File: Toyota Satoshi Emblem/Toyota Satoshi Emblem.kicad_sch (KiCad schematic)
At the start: 293 parts

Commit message: v1.1
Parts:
- removed D? (x58): W_LED, symbol Device:LED
- removed J?: Conn_01x20_Male, symbol Connector:Conn_01x20_Male
- removed Q? (x6): BC337, Package_TO_SOT_THT:TO-92_Inline, symbol Transistor_BJT:BC337
- removed Q? (x12): BC327, Package_TO_SOT_THT:TO-92_Inline, symbol Transistor_BJT:BC327
- removed R? (x29): 10Ω, symbol Device:R
- removed R? (x12): 10KΩ, symbol Device:R
- removed R? (x12): 200Ω, symbol Device:R
- added D? (x86): A_LED, symbol Device:LED
- added Q? (x6): BC327, Package_TO_SOT_THT:TO-92_Inline, symbol Transistor_BJT:BC327
- added Q? (x12): S8550, Package_TO_SOT_THT:TO-92_Inline, symbol Transistor_BJT:S8550
- added R? (x86): 9Ω, symbol Device:R
- added R? (x12): 200Ω, symbol Device:R
- added R? (x12): 10KΩ, symbol Device:R
- added U? (x7): 74HC04, symbol 74xx:74HC04
- R?: value 200Ω -> 7.5k
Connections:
- net +5V: now also R?.2, R?.2, R?.2, R?.2, R?.2, R?.2, R?.2, R?.2, R?.2, R?.2, R?.2, R?.2
- net BUCK_A: now also Q?.3 (E), Q?.3 (E), Q?.3 (E)
- net BUCK_B: now also Q?.3 (E), Q?.3 (E), Q?.3 (E)
- net GND: now also D?.1 (K), D?.1 (K), D?.1 (K), D?.1 (K), D?.1 (K), D?.1 (K), D?.1 (K), D?.1 (K), D?.1 (K), D?.1 (K), D?.1 (K), D?.1 (K), D?.1 (K), D?.1 (K), D?.1 (K), D?.1 (K), D?.1 (K), D?.1 (K), D?.1 (K), D?.1 (K), D?.1 (K), D?.1 (K), D?.1 (K), D?.1 (K), D?.1 (K), D?.1 (K), D?.1 (K), D?.1 (K), D?.1 (K), D?.1 (K), D?.1 (K), D?.1 (K), D?.1 (K), D?.1 (K), D?.1 (K), D?.1 (K), D?.1 (K), D?.1 (K), D?.1 (K), D?.1 (K), D?.1 (K), D?.1 (K), D?.1 (K), D?.1 (K), D?.1 (K), D?.1 (K), D?.1 (K), D?.1 (K), D?.1 (K), D?.1 (K), D?.1 (K), D?.1 (K), D?.1 (K), D?.1 (K), D?.1 (K), D?.1 (K), D?.1 (K), D?.1 (K), D?.1 (K), D?.1 (K), D?.1 (K), D?.1 (K), D?.1 (K), D?.1 (K), D?.1 (K), D?.1 (K), D?.1 (K), D?.1 (K), D?.1 (K), D?.1 (K), D?.1 (K), D?.1 (K), R?.1, R?.1, R?.1, R?.1, R?.1, R?.1; no longer R?.2, R?.2, R?.2, R?.2, R?.2, R?.2
- net at R?.1, R?.1, R?.1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: now also Q?.3 (C)
- net at R?.2: now also U?.4
- net at R?.1, R?.1, R?.1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: now also Q?.3 (C) (x2)
- net at R?.1, R?.1: now also Q?.2 (B) (x6)
- net at R?.1, R?.1, R?.1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: now also Q?.3 (C), R?.1
- net at R?.1, R?.1, R?.1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: now also Q?.3 (C), R?.1, R?.1 (x2)
- net at R?.2: now also U?.6
- net at R?.2: now also U?.8
- net at R?.2: now also U?.2
- net at R?.2: now also U?.12
- net at R?.2: now also U?.10
- new net: D?.1 (K), D?.2 (A) (x43)
- new net: D?.2 (A), R?.2 (x43)
- new net: R?.2, U?.3
- new net: R?.1, R?.2 (x43)
- new net: Q?.2 (B), R?.2, R?.2 (x6)
- new net: Q?.1 (E), Q?.1 (E) (x6)
- new net: Q?.2 (B), R?.1, R?.1 (x6)
- new net: Q?.3 (C), R?.1, R?.1, R?.1, R?.1, R?.1, R?.1 (x5)
- new net: R?.2, U?.9
- new net: R?.2, U?.1
- new net: R?.2, U?.11
- new net: R?.2, U?.5
- new net: Q?.3 (C), R?.1, R?.1, R?.1, R?.1
- new net: R?.2, U?.13
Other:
- note removed: "WHITE"
- note removed: "WHITE TOGGLE"
- moved on the sheet: D?, R?

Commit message: v1.2
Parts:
- removed Q? (x6): BC327, Package_TO_SOT_THT:TO-92_Inline, symbol Transistor_BJT:BC327
- removed Q? (x12): S8550, Package_TO_SOT_THT:TO-92_Inline, symbol Transistor_BJT:S8550
- removed R? (x17): 200Ω, symbol Device:R
- removed R? (x36): 9Ω, symbol Device:R
- removed R? (x18): 10KΩ, symbol Device:R
- removed R?: 7.5k, symbol Device:R
- removed U? (x7): 74HC04, symbol 74xx:74HC04
- added Q? (x6): 2N3904, Package_TO_SOT_THT:TO-92_Inline, symbol Transistor_BJT:2N3904
- added Q? (x18): IRLZ44N, Package_TO_SOT_THT:TO-220-3_Vertical, symbol Transistor_FET:IRLZ44N
- added R? (x12): 10K, symbol Device:R
- added R? (x6): 200, symbol Device:R
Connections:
- net at R?.1, R?.1, R?.1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: now also R?.1, R?.1, Q?.2 (D) (x2)
- net at R?.2: now also D?.2 (A) (x26)
- net at D?.2 (A): now also R?.2 (x10)
- net at R?.1, R?.1, R?.1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: now also Q?.2 (D) (x10)
- new net: Q?.1 (G), Q?.3 (C), R?.1 (x6)
- new net: R?.2, R?.2 (x3)
- new net: Q?.1 (E), Q?.3 (S), R?.2 (x6)
- new net: Q?.2 (B), R?.1 (x6)
- new net: Q?.2 (D), Q?.3 (S), Q?.3 (S) (x6)
- new net: Q?.1 (G), R?.1, R?.2 (x6)
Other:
- note removed: "AMBER TOGGLE"
- note removed: "LETTER INTENSITY"
- moved on the sheet: D?, R?

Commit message: v1.3
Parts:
- removed D? (x120): A_LED, symbol Device:LED
- removed J?: Conn_01x20_Female, symbol Connector:Conn_01x20_Female
- removed R? (x90): 9Ω, symbol Device:R
- added C?: 200uF, symbol Device:C_Polarized
- added C?: 100uF, symbol Device:C_Polarized
- added D? (x120): A_LED, symbol Device:LED
- added D?: 1N5822, Diode_THT:D_DO-201AD_P15.24mm_Horizontal, symbol Diode:1N5822
- added J? (x6): Conn_01x03_Male, symbol Connector:Conn_01x03_Male
- added J? (x6): Letter Terminal, symbol Connector:Conn_01x03_Female
- added L?: 68uH, symbol Device:L
- added R? (x2): R, symbol Device:R
- added R? (x90): 9Ω, symbol Device:R
- added U?: LM2596S-ADJ, Package_TO_SOT_SMD:TO-263-5_TabPin3, symbol Regulator_Switching:LM2596S-ADJ
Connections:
- net BUCK_A: now also R?.2, R?.2, J?.2 (Pin_2), J?.2 (Pin_2)
- net BUCK_B: now also R?.2, R?.2, J?.2 (Pin_2), J?.2 (Pin_2)
- net GND: now also Q?.1 (E), Q?.1 (E), Q?.1 (E), Q?.1 (E), Q?.1 (E), Q?.1 (E), Q?.3 (S), Q?.3 (S), Q?.3 (S), Q?.3 (S), Q?.3 (S), Q?.3 (S), R?.2, R?.2, R?.2, R?.2, R?.2, R?.2, C?.2, C?.2, D?.2 (A), R?.1, U?.3 (GND); no longer A?.4 (GND), D?.1 (K), D?.1 (K), D?.1 (K), D?.1 (K), D?.1 (K), D?.1 (K), D?.1 (K), D?.1 (K), D?.1 (K), D?.1 (K), D?.1 (K), D?.1 (K)
- net VDD: now also C?.1, U?.1 (VIN)
- net at Q?.2 (D): now also J?.1 (Pin_1) (x5)
- net BUCK_C: now reaches R?.2, R?.2
- net BUCK_C: now also C?.1, J?.2 (Pin_2), J?.2 (Pin_2), L?.2, R?.1
- net at Q?.1 (G): now also A?.13 (D10)
- net at Q?.1 (G), R?.1, R?.2: now also A?.11 (D8)
- net at R?.1, R?.1, R?.1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: now also R?.1, R?.1, R?.1, R?.1, R?.1, R?.1, J?.2 (Pin_2); no longer Q?.2 (D)
- net at Q?.1 (G), R?.1, R?.2: now also A?.5 (D2)
- net at Q?.2 (D): now also J?.3 (Pin_3) (x5)
- net at Q?.1 (G): now also A?.6 (D3)
- net at A?.15 (D12): now also Q?.1 (G), R?.1, R?.2
- net at A?.16 (D13): now also Q?.1 (G), R?.1, R?.2
- net at A?.8 (D5): now also Q?.1 (G)
- net at A?.9 (D6): now also Q?.1 (G)
- net at A?.12 (D9): now also Q?.1 (G)
- net at A?.14 (D11): now also Q?.1 (G)
- net at A?.7 (D4): now also Q?.1 (G), R?.1, R?.2
- net at A?.10 (D7): now also Q?.1 (G), R?.1, R?.2
- new net: D?.1 (K), D?.2 (A) (x60)
- new net: D?.2 (A), R?.2 (x60)
- new net: D?.1 (K), D?.1 (K), D?.1 (K), D?.1 (K), D?.1 (K), D?.1 (K), J?.1 (Pin_1) (x6)
- new net: J?.2 (Pin_2), R?.1, R?.1, R?.1, R?.1, R?.1, R?.1, R?.1, R?.1, R?.1, R?.1, R?.1, R?.1 (x5)
- new net: D?.1 (K), D?.1 (K), D?.1 (K), D?.1 (K), D?.1 (K), D?.1 (K), J?.3 (Pin_3) (x6)
- new net: R?.2, R?.2, U?.4 (FB)
- new net: R?.1, R?.2 (x30)
- new net: J?.1 (Pin_1), Q?.2 (D)
- new net: J?.3 (Pin_3), Q?.2 (D)
- new net: D?.1 (K), L?.1, U?.2 (OUT)
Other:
- note removed: "AMBER"
- moved on the sheet: 5A, 6A10, A?, C?, D?, L?, Q?, R?, U?

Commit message: v1.4
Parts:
- removed Q?: BC327, Package_TO_SOT_THT:TO-92_Inline, symbol Transistor_BJT:BC327
- removed R? (x60): 9Ω, symbol Device:R
- added C?: 0.22u, symbol Device:C
- added D? (x4): 1N47xxA, Diode_THT:D_DO-41_SOD81_P10.16mm_Horizontal, symbol Diode:1N47xxA
- added J?: Power Port Terminal, symbol Connector_Generic:Conn_02x04_Counter_Clockwise
- added J? (x2): Serial Terminal, symbol Connector:Conn_01x02_Male
- added J?: Ambient Harness, symbol Connector:Conn_01x02_Female
- added K?: FINDER-40.51, Relay_THT:Relay_SPDT_Finder_40.51, symbol Relay:FINDER-40.51
- added Q?: BC337, Package_TO_SOT_THT:TO-92_Inline, symbol Transistor_BJT:BC337
- added R? (x60): 8.2, symbol Device:R
- added R? (x7): 10K, symbol Device:R
- added R?: R_Photo, symbol Device:R_Photo
- added R? (x4): 1K, symbol Device:R
- C?: value C_Polarized -> 10u
- C?: value C_Polarized -> 4.7u
- C?: value C -> 0.1u
- D?: value 5KPxxA -> 5KP16A
- F?: renamed from 5A; value Fuse -> 7.5A
- L? (x3): value 68uH -> 47uH
- R? (x12): value 9Ω -> 8.2
- R? (x36): value 9Ω -> 3.3
- R?: value R -> 1K
- R? (x6): value 200 -> 1K
- R? (x2): value R -> 3.3K
- R?: value R -> 4.7K
- R? (x2): value R -> 1.5K
- R?: value R -> 10K
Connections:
- net +5VD is gone; now on net +5V: C?.1, C?.1, U?.3 (OUT)
- net VDD is gone; now on net +12V: C?.1, C?.1, C?.1, U?.1 (VIN), U?.1 (VIN), U?.1 (VIN)
- net BUCK_A: now also J?.1 (Pin_1), R?.2, R?.2
- net BUCK_B: now also J?.2 (Pin_2), R?.2, R?.2
- net BUCK_C: now also J?.8 (Pin_8), R?.2, R?.2
- net GND: now also A?.29 (GND), C?.2, D?.2 (A), D?.2 (A), D?.2 (A), D?.2 (A), J?.1 (Pin_1), J?.4 (Pin_4), J?.5 (Pin_5), K?.A1
- net at D?.2 (A): now also R?.2 (x30)
- net at J?.2 (Pin_2), R?.1, R?.1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: now also R?.1, R?.1, R?.1, R?.1, R?.1, R?.1 (x5)
- net at A?.13 (D10), Q?.1 (G): now also R?.1
- net at 6A10.1 (K), C?.1, D?.1 (A1)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: now also C?.1, Q?.1 (C)
- net at A?.6 (D3), Q?.1 (G): now also R?.1
- net at F?.1: now also 6A10.2 (A)
- net at F?.2: now also K?.14; no longer 6A10.2 (A)
- net at A?.12 (D9), Q?.1 (G): now also R?.1
- net at R?.2: now also Q?.2 (B)
- net at D?.2 (A): now also Q?.3 (E)
- net at A?.9 (D6), Q?.1 (G): now also R?.1
- net at A?.1 (D1/TX): now also J?.2 (Pin_2)
- net at A?.14 (D11), Q?.1 (G): now also R?.1
- net at A?.2 (D0/RX): now also D?.1 (K), R?.1
- net at A?.23 (A4): now also D?.1 (K), R?.2
- net at A?.24 (A5): now also D?.1 (K), R?.2
- net at A?.25 (A6): now also D?.1 (K), R?.2
- net at A?.26 (A7): now also J?.2 (Pin_2), R?.2
- net +5V: now reaches A?.27 (+5V)
- net +5V: now also J?.7 (Pin_7), R?.1
- net at A?.8 (D5), Q?.1 (G): now also R?.1
- net VD renamed +12V
- net +12V: now also J?.3 (Pin_3), J?.6 (Pin_6)
- new net: R?.1, R?.2 (x30)
- new net: J?.1 (Pin_1), R?.1
- new net: J?.2 (Pin_2), R?.2
- new net: J?.1 (Pin_1), R?.2
- new net BAT +12V: K?.11
- new net HEAD RLY (R-B): K?.A2
- new net L Turn Sig: R?.1
- new net R Turn Sig: R?.1
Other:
- note added: "VEHICLE POWER ----->"
- moved on the sheet: 6A10, A?, C?, D?, F?, J?, L?, Q?, R?, U?

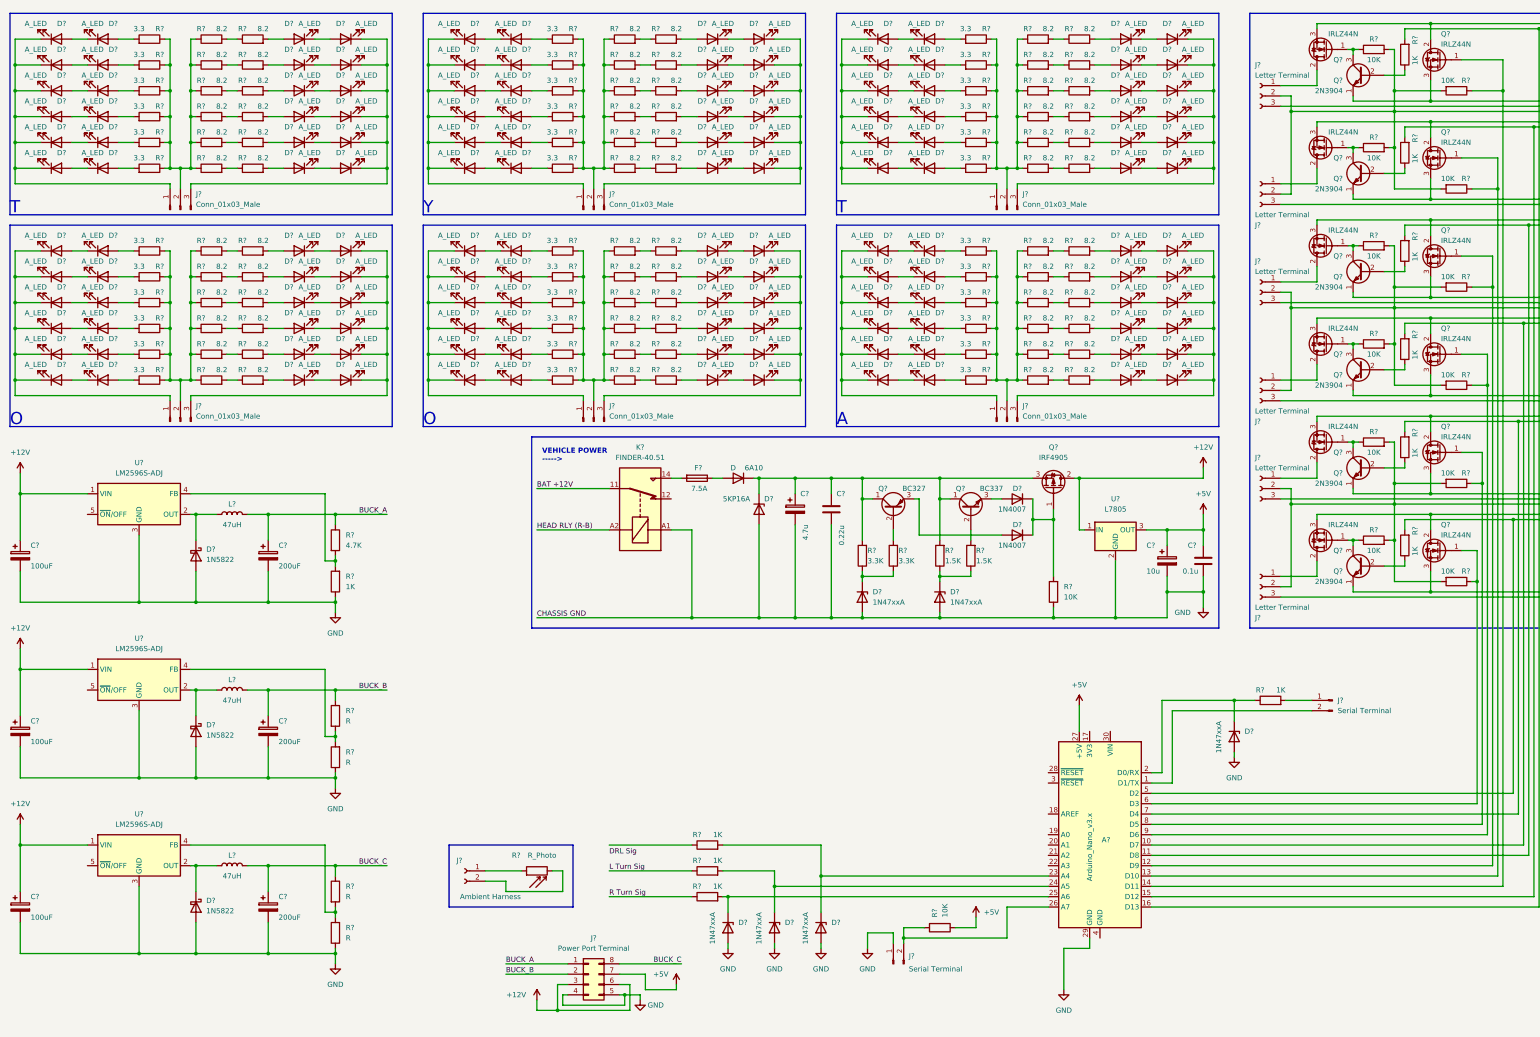
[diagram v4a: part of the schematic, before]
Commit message: v1.5
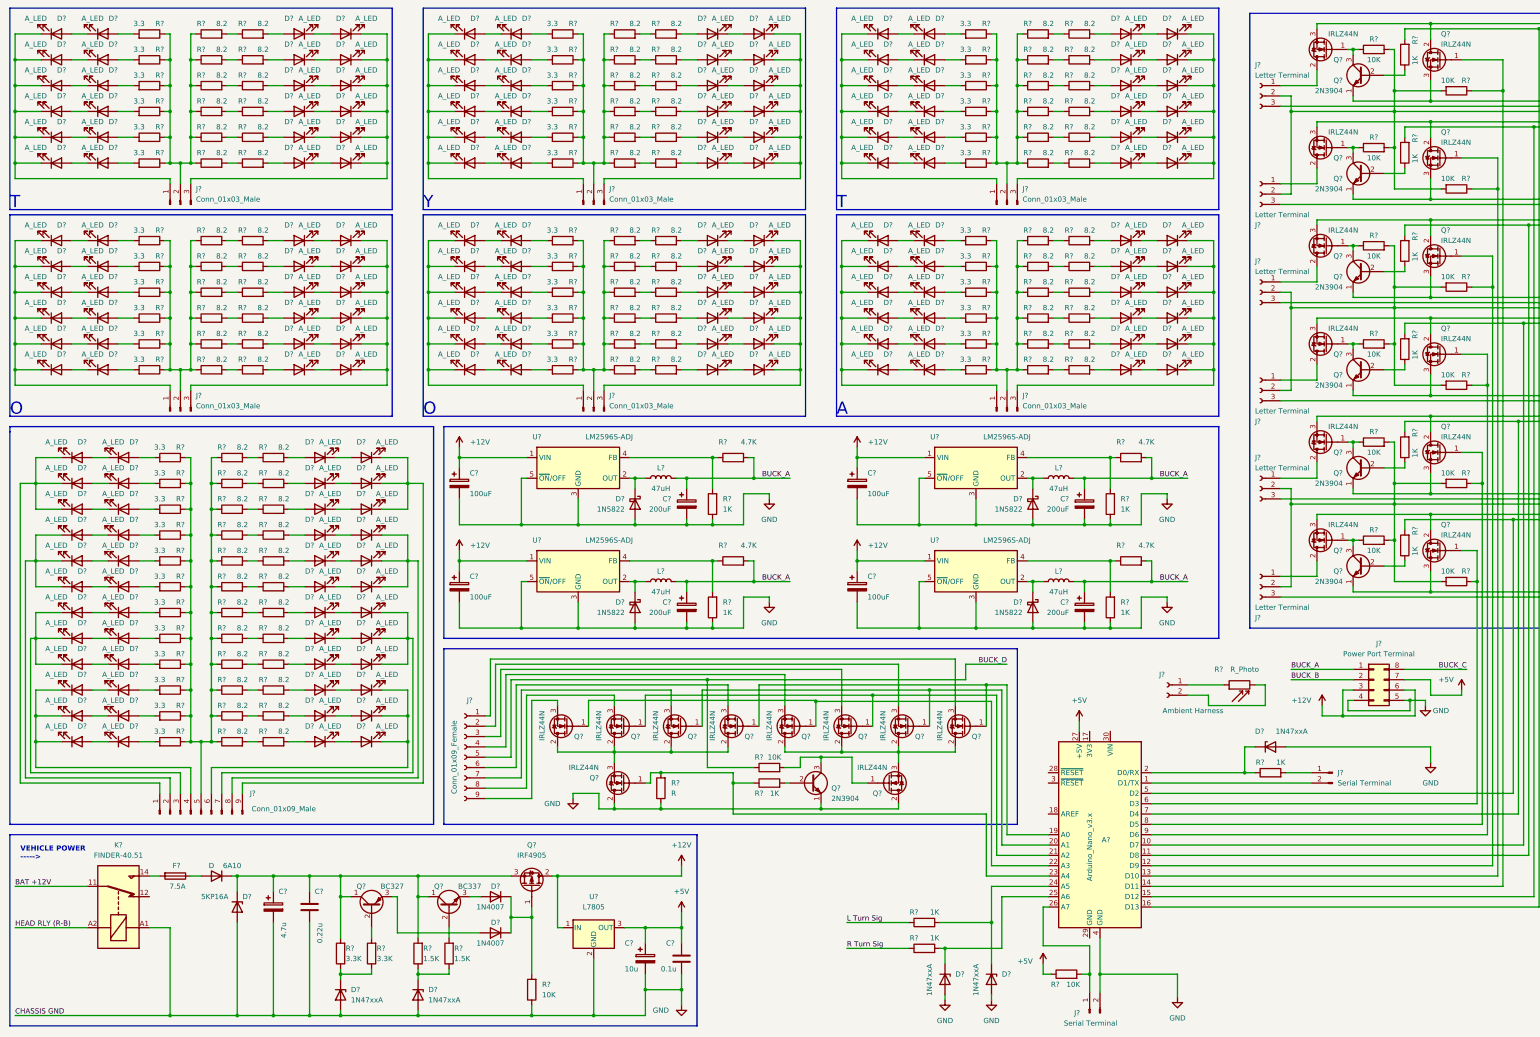
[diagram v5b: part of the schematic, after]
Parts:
- removed C? (x3): 200uF, symbol Device:C_Polarized
- removed C? (x3): 100uF, symbol Device:C_Polarized
- removed D?: 1N47xxA, Diode_THT:D_DO-41_SOD81_P10.16mm_Horizontal, symbol Diode:1N47xxA
- removed D? (x3): 1N5822, Diode_THT:D_DO-201AD_P15.24mm_Horizontal, symbol Diode:1N5822
- removed L? (x3): 47uH, symbol Device:L
- removed R? (x4): R, symbol Device:R
- removed R? (x2): 1K, symbol Device:R
- removed R?: 4.7K, symbol Device:R
- removed U? (x3): LM2596S-ADJ, Package_TO_SOT_SMD:TO-263-5_TabPin3, symbol Regulator_Switching:LM2596S-ADJ
- added C? (x4): 200uF, symbol Device:C_Polarized
- added C? (x4): 100uF, symbol Device:C_Polarized
- added D? (x48): A_LED, symbol Device:LED
- added D? (x4): 1N5822, Diode_THT:D_DO-201AD_P15.24mm_Horizontal, symbol Diode:1N5822
- added J?: Conn_01x09_Male, symbol Connector:Conn_01x09_Male
- added J?: Conn_01x09_Female, symbol Connector:Conn_01x09_Female
- added L? (x4): 47uH, symbol Device:L
- added Q?: 2N3904, Package_TO_SOT_THT:TO-92_Inline, symbol Transistor_BJT:2N3904
- added Q? (x10): IRLZ44N, Package_TO_SOT_THT:TO-220-3_Vertical, symbol Transistor_FET:IRLZ44N
- added R? (x24): 8.2, symbol Device:R
- added R? (x12): 3.3, symbol Device:R
- added R?: 10K, symbol Device:R
- added R? (x5): 1K, symbol Device:R
- added R?: R, symbol Device:R
- added R? (x4): 4.7K, symbol Device:R
- added U? (x4): LM2596S-ADJ, Package_TO_SOT_SMD:TO-263-5_TabPin3, symbol Regulator_Switching:LM2596S-ADJ
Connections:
- net +12V: now also C?.1, C?.1, C?.1, C?.1, U?.1 (VIN), U?.1 (VIN), U?.1 (VIN), U?.1 (VIN)
- net BUCK_A: now also C?.1, C?.1, C?.1, C?.1, L?.2, L?.2, L?.2, L?.2, R?.2, R?.2, R?.2, R?.2
- net GND: now also A?.4 (GND), J?.2 (Pin_2), C?.2, C?.2, C?.2, C?.2, C?.2, C?.2, C?.2, C?.2, D?.2 (A), D?.2 (A), D?.2 (A), D?.2 (A), Q?.1 (E), Q?.2 (D), Q?.2 (D), R?.1, R?.1, R?.1, R?.1, R?.1, U?.3 (GND), U?.3 (GND), U?.3 (GND), U?.3 (GND), U?.5 (~{ON}/OFF), U?.5 (~{ON}/OFF), U?.5 (~{ON}/OFF), U?.5 (~{ON}/OFF); no longer A?.29 (GND), J?.1 (Pin_1)
- net at A?.23 (A4): now also Q?.1 (G), R?.1, R?.2
- net at A?.26 (A7), R?.2: now also J?.1 (Pin_1); no longer J?.2 (Pin_2)
- net at A?.19 (A0): now also Q?.1 (G), Q?.1 (G)
- net at A?.20 (A1): now also Q?.1 (G), Q?.1 (G)
- net at A?.21 (A2): now also Q?.1 (G), Q?.1 (G)
- net at A?.22 (A3): now also Q?.1 (G), Q?.1 (G)
- new net: R?.1, R?.2 (x12)
- new net: D?.2 (A), R?.2 (x24)
- new net: D?.1 (K), L?.1, U?.2 (OUT) (x4)
- new net: R?.1, R?.2, U?.4 (FB) (x4)
- new net: D?.1 (K), D?.1 (K), D?.1 (K), J?.1 (Pin_1)
- new net: D?.1 (K), D?.2 (A) (x24)
- new net: J?.5 (Pin_5), R?.1, R?.1, R?.1, R?.1, R?.1, R?.1, R?.1, R?.1, R?.1, R?.1, R?.1, R?.1, R?.1, R?.1, R?.1, R?.1, R?.1, R?.1, R?.1, R?.1, R?.1, R?.1, R?.1, R?.1
- new net: D?.1 (K), D?.1 (K), D?.1 (K), J?.2 (Pin_2)
- new net: D?.1 (K), D?.1 (K), D?.1 (K), J?.3 (Pin_3)
- new net: D?.1 (K), D?.1 (K), D?.1 (K), J?.4 (Pin_4)
- new net: D?.1 (K), D?.1 (K), D?.1 (K), J?.6 (Pin_6)
- new net: D?.1 (K), D?.1 (K), D?.1 (K), J?.7 (Pin_7)
- new net: D?.1 (K), D?.1 (K), D?.1 (K), J?.8 (Pin_8)
- new net: D?.1 (K), D?.1 (K), D?.1 (K), J?.9 (Pin_9)
- new net: Q?.1 (G), Q?.3 (C), R?.2
- new net: Q?.2 (B), R?.2
- new net: Q?.2 (D), Q?.2 (D), Q?.2 (D), Q?.2 (D), Q?.3 (S) (x2)
- new net: J?.7 (Pin_7), Q?.3 (S)
- new net: J?.1 (Pin_1), Q?.3 (S)
- new net: J?.3 (Pin_3), Q?.3 (S)
- new net: J?.8 (Pin_8), Q?.3 (S)
- new net: J?.4 (Pin_4), Q?.3 (S)
- new net: J?.2 (Pin_2), Q?.3 (S)
- new net: J?.9 (Pin_9), Q?.3 (S)
- new net: J?.6 (Pin_6), Q?.3 (S)
- new net BUCK_D: J?.5 (Pin_5), R?.1
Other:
- moved on the sheet: 6A10, C?, D?, F?, J?, K?, Q?, R?, U?
